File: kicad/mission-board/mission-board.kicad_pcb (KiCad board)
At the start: 2 copper layers, 100 x 74 mm, 126 parts, among them J1 Servo 1, J10 MOSFET Ch2 Out, J11 MOSFET Ch3 Out, J12 MOSFET Ch4 Out, J13 Camera FPC, J14 I2C Expansion, J15 SPI Expansion, J16 GPIO/ADC Expansion, J17 Debug UART, J18 Inter-ESP UART, J19 Servo 5, J2 Servo 2, J20 Servo 6, J21 Fast IO Expansion, J22 Limit Switch Input, J23 H-Bridge Ch Out, J24 H-Bridge Ch Out, J25 H-Bridge Ch Out, J26 H-Bridge Ch Out, J3 Servo 3, J4 Servo 4, J5 USB-C, J6 Actuator Power In (5-6V BEC O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, J7 H-Bridge Ch Out, J8 H-Bridge Ch Out, J9 MOSFET Ch1 Out, Q1 reverse polarity protection, Q2 AO3400A, Q3 AO3400A, Q4 AO3400A, Q5 AO3400A, SW1 TS-1088, SW2 TS-1088, U1 INA180A2IDBVR, U10 24MHz Oscillator, U11 ESP32-S3-WROOM-1, U12 PCA9685PW, U13 DRV8833, U14 DRV8833, U15 USBLC6-2SC6, U16 XC6206P282MR, U17 XC6206P122MR, U18 PCA9685PW, U2 XC6220B331PR-G, U3 DRV8833, U4 INA180A2IDBVR, U5 INA180A2IDBVR, U6 INA180A2IDBVR, U7 INA180A2IDBVR, U8 MCP23017, U9 CD74HC4067

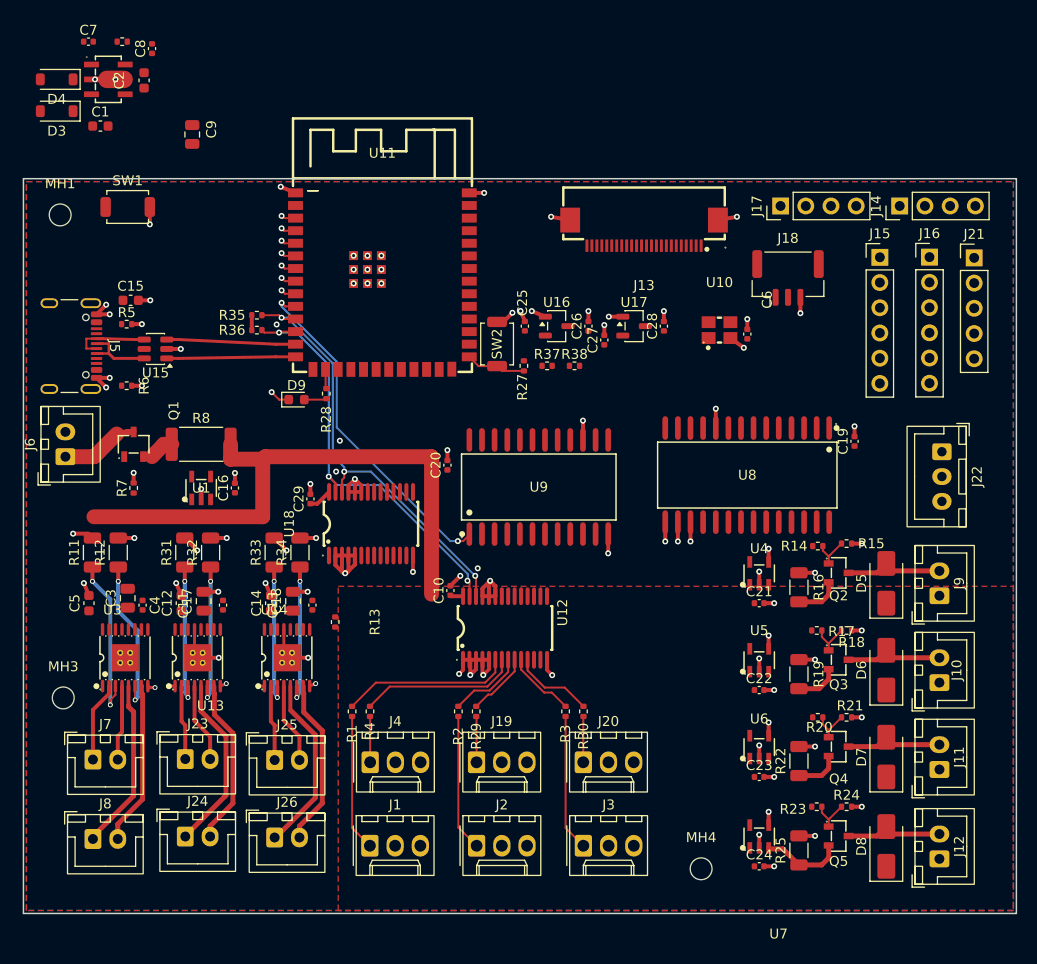
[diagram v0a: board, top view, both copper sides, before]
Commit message: Kicad FC v3.1 complete, Mission Controller and UWB boards v1 complete, firmware v2 complete!
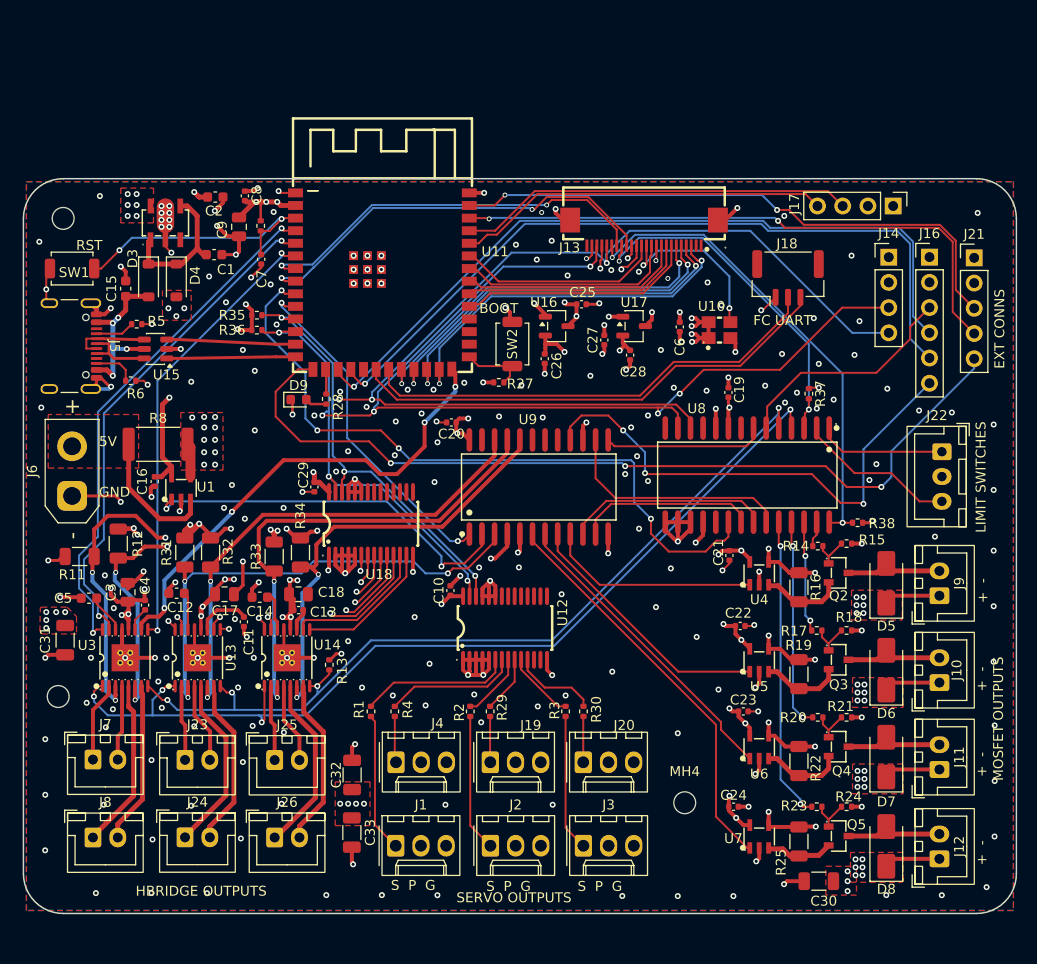
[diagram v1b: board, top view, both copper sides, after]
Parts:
- removed J15: SPI Expansion, Connector_PinHeader_2.54mm:PinHeader_1x06_P2.54mm_Vertical
- removed Q1: reverse polarity protection, easyeda2kicad:SOT-23-3_L2.9-W1.6-P1.90-LS2.8-BR
- removed R7: 100K, Resistor_SMD:R_0402_1005Metric
- added C30: 47uF, Capacitor_SMD:C_1206_3216Metric, F.Cu at (141.6, 146.5)
- added C31: 47uF, Capacitor_SMD:C_1206_3216Metric, F.Cu at (65.7, 122.2)
- added C32: 47uF, Capacitor_SMD:C_1206_3216Metric, F.Cu at (94.6, 135.8)
- added C33: 47uF, Capacitor_SMD:C_1206_3216Metric, F.Cu at (94.6, 141.6)
- added G***: LOGO, LOGO, B.Cu at (122.8, 119.0)
- C17, C18, C3, C9: value 10uF -> 22uF
- J6: value Actuator Power In (5-6V BEC ONLY) -> Actuator Power In; footprint Connector_JST:JST_XH_B2B-XH-A_1x02_P2.50mm_Vertical -> Connector_AMASS:AMASS_XT30UPB-M_1x02_P5.0mm_Vertical
- R8: value 0.02R -> 0.005R
- moved R38 32.6 mm to (145.5, 110.4), turned to 180 degrees
- moved C7 28.0 mm to (85.4, 83.9), turned to -90 degrees
- moved R37 26.5 mm to (140.6, 97.4), turned to -90 degrees
- moved D4 23.6 mm to (76.9, 86.0), turned to -90 degrees
- moved R26 23.2 mm to (85.4, 80.5), turned to 90 degrees
- moved D3 19.4 mm to (74.1, 86.0), turned to -90 degrees
- moved C8 17.5 mm to (83.8, 77.5)
- moved C1 17.3 mm to (80.7, 83.4)
- moved U2 15.6 mm to (75.8, 80.2), turned to -90 degrees
- moved C2 13.8 mm to (80.8, 77.6), turned to 0 degrees
- moved C19 13.6 mm to (132.5, 97.3)
- moved J17 11.3 mm to (149.1, 78.5), turned to -90 degrees
- moved C9 10.4 mm to (83.2, 80.6), turned to -90 degrees
- moved SW1 8.35 mm to (66.4, 84.8), turned to 180 degrees
- moved C16 8.10 mm to (74.7, 106.2), turned to -90 degrees
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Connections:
- J16 pad 4: unconnected-(J16-Pin_4-Pad4) -> /FASTIO4
- J16 pad 5: unconnected-(J16-Pin_5-Pad5) -> /FASTIO5
- J18 pad 1: /INTER_ESP_UART_TX -> /GND
- J18 pad 3: /GND -> /INTER_ESP_UART_TX
- J6 pad 1: /power/BATT_IN -> /GND
- J6 pad 2: /GND -> /power/ACT_PWR_PRESHUNT
- U11 pad 17: /SPI_SCK -> /FASTIO4
- U11 pad 18: /SPI_MISO -> /FASTIO5
- U11 pad 19: /SPI_MOSI -> unconnected-(U11-IO11-Pad19)
- U11 pad 20: /INTER_ESP_UART_RX -> /INTER_ESP_UART_TX
- U11 pad 21: /INTER_ESP_UART_TX -> /INTER_ESP_UART_RX
- U11 pad 22: /CAM_D2 -> /CAM_D0
- U11 pad 23: /CAM_D1 -> /CAM_D3
- U11 pad 24: /CAM_D3 -> /CAM_D1
- U11 pad 25: /CAM_D0 -> /CAM_D2
- U18 pad 12: /HBRIDGE3_BIN1 -> /HBRIDGE3_BIN2
- U18 pad 13: /HBRIDGE3_BIN2 -> /HBRIDGE3_BIN1
- U18 pad 8: /HBRIDGE2_BIN1 -> /HBRIDGE2_BIN2
- U18 pad 9: /HBRIDGE2_BIN2 -> /HBRIDGE2_BIN1
- U8 pad 1: /expander_mux/MUX_S0 -> /expander_mux/LIMIT_SW1
- U8 pad 2: /expander_mux/MUX_S1 -> /expander_mux/LIMIT_SW2
- U8 pad 21: /MOSFET1_GATE -> /expander_mux/MUX_S1
- U8 pad 22: /MOSFET2_GATE -> /expander_mux/MUX_S0
- U8 pad 23: /MOSFET3_GATE -> /expander_mux/MUX_S2
- U8 pad 25: /HBRIDGE_NSLEEP -> /MOSFET3_GATE
- U8 pad 26: /HBRIDGE_NFAULT -> /MOSFET2_GATE
- U8 pad 27: /CAM_PWDN -> /MOSFET1_GATE
- U8 pad 3: /expander_mux/MUX_S2 -> /CAM_PWDN
- U8 pad 4: /expander_mux/MUX_S3 -> /HBRIDGE_NSLEEP
- U8 pad 5: /expander_mux/LIMIT_SW2 -> /HBRIDGE_NFAULT
- U8 pad 7: /expander_mux/LIMIT_SW1 -> /expander_mux/MUX_S3
- U8 pad 8: /SPI_CS -> unconnected-(U8-GPB7-Pad8)
- U9 pad 16: unconnected-(U9-I15-Pad16) -> /EXP_ADC
- U9 pad 23: /EXP_ADC -> unconnected-(U9-I8-Pad23)
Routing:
- net /I2C_SCL: track 43.8 -> 149.7 mm, vias 3 -> 6
- net /I2C_SDA: track 43.1 -> 141.2 mm, vias 3 -> 8
- net /HBRIDGE_NSLEEP: track 1.30 -> 96.6 mm, vias 2 -> 4
- net /esp32_core/FASTIO3: track 0.00 -> 87.9 mm, vias 0 -> 3
- net /HBRIDGE_NFAULT: track 2.15 -> 86.6 mm, vias 3 -> 4
- net /GND: track 140.5 -> 219.8 mm, vias 93 -> 247
- net /ESP_3V3: track 5.19 -> 82.7 mm, vias 0 -> 42
- net /FASTIO5: track 0.00 -> 77.0 mm, vias 0 -> 1
- net /FASTIO4: track 0.00 -> 76.5 mm, vias 0 -> 1
- net /MCP_INT: track 1.54 -> 71.0 mm, vias 1 -> 4
- net /esp32_core/FASTIO2: track 0.00 -> 60.0 mm, vias 0 -> 2
- net /esp32_core/FASTIO1: track 0.00 -> 58.9 mm, vias 0 -> 2
- net /EXP_ADC: track 0.00 -> 51.1 mm, vias 0 -> 3
- net /HBRIDGE_AIN1: track 1.50 -> 52.4 mm, vias 1 -> 2
- net /HBRIDGE_AISENSE: track 16.7 -> 66.5 mm, vias 2 -> 4
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- added copper zone on In2.Cu, net /ACT_PWR
- added copper zone on F.Cu, net /ESP_3V3
- added copper zone on In2.Cu, net /ESP_3V3
- added copper zone on In1.Cu, net /GND
- added copper zone on F.Cu, net /power/ACT_PWR_PRESHUNT
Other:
- outline, holes or cut-outs redrawn
- copper layers 2 -> 4
- board text added: "+ -"
- board text added: "5V"
- board text added: "BOOT"
- board text added: "EXT CONNS"
- board text added: "FC UART"
- board text added: "GND"
- board text added: "HBRIDGE OUTPUTS"
- board text added: "LIMIT SWITCHES"
- board text added: "MOSFET OUTPUTS"
- board text added: "Mission Board v1.0 TMB October 2026"
- board text added: "RST"
- board text added: "S P G"
- board text added: "SERVO OUTPUTS"
